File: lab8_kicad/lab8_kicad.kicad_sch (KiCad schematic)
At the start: 24 parts, among them J1 Command Generator, M1 Motor, SW1 Reset, U1 SN754410, U2 PIC32MX170F256B

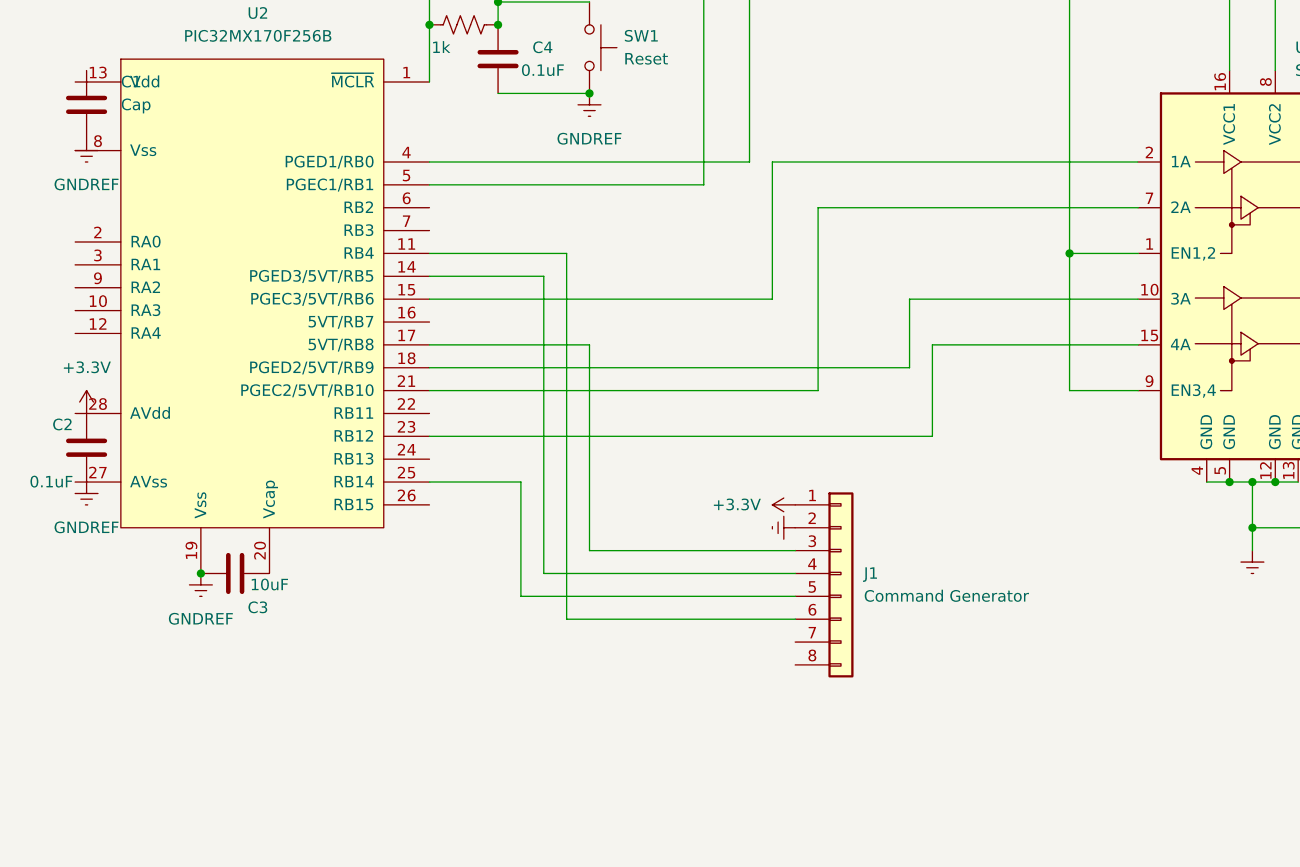
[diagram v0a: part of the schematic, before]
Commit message: suibian
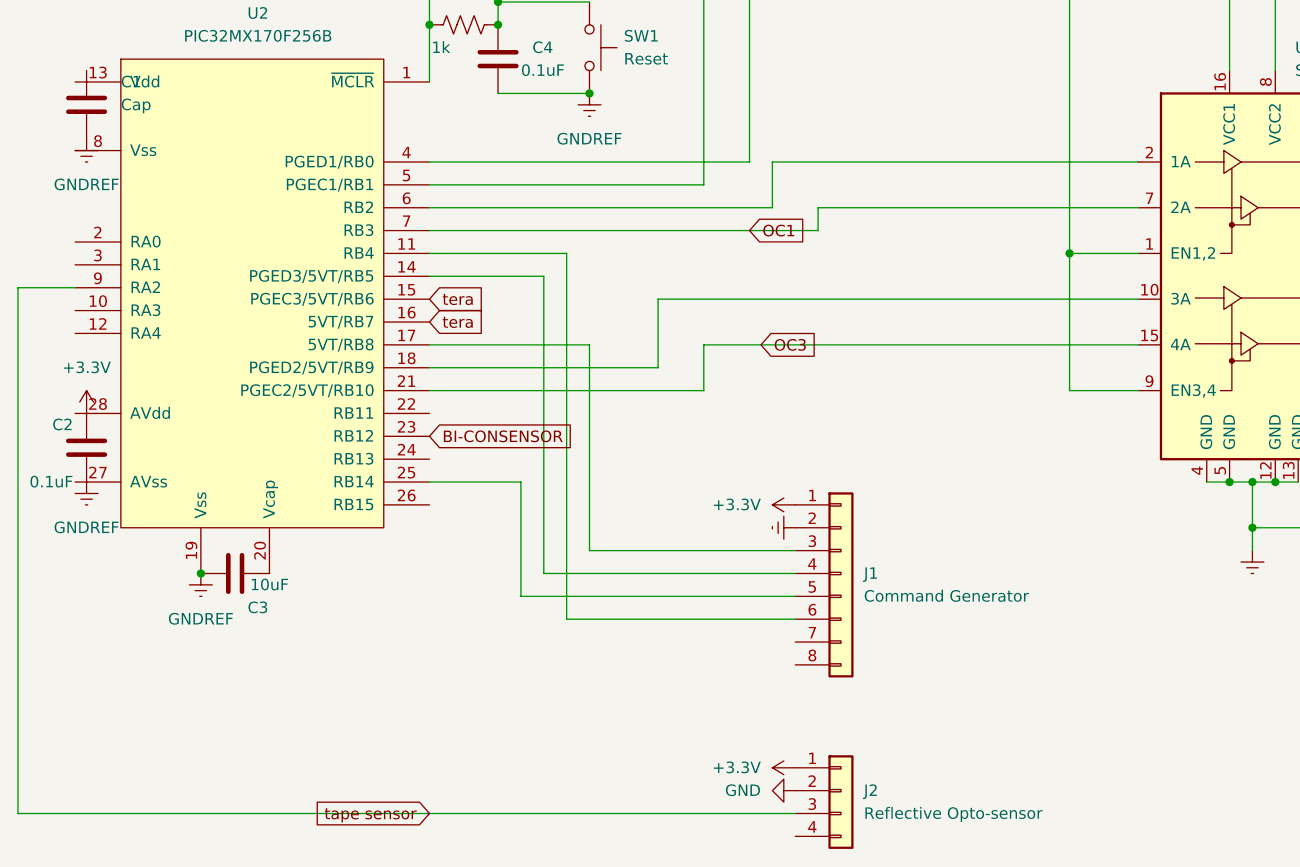
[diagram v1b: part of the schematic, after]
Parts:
- added J2: Reflective Opto-sensor, symbol ME218_BaseLib:Molex4
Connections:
- net +3.3V: now also J2.1 (Pin_1)
- net GND: now also J2.2 (Pin_2)
- net BI-CONSENSOR: now reaches U2.23 (RB12)
- net BI-CONSENSOR: no longer U1.15 (4A)
- net at U1.2 (1A): now also U2.6 (RB2); no longer U2.15 (PGEC3/5VT/RB6)
- net OC1: now reaches U1.7 (2A)
- net OC1: now also U2.7 (RB3); no longer U2.21 (PGEC2/5VT/RB10)
- net tera: now reaches U2.16 (5VT/RB7)
- net tera: now also U2.15 (PGEC3/5VT/RB6)
- net tape sensor: now reaches U2.9 (RA2)
- net tape sensor: now also J2.3 (Pin_3)
- new net OC3: U1.15 (4A), U2.21 (PGEC2/5VT/RB10)
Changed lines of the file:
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@@
+    (stroke (width 0) (type default))
+  )
+  (wire (pts (xy 104.14 60.96) (xy 66.04 60.96))
+    (stroke (width 0) (type default))
+  )
+  (wire (pts (xy 104.14 55.88) (xy 104.14 60.96))
     (stroke (width 0) (type default))
   )
@@
     (stroke (width 0) (type default))
   )
-  (wire (pts (xy 104.14 55.88) (xy 104.14 71.12))
-    (stroke (width 0) (type default))
-  )
   (wire (pts (xy 210.82 38.1) (xy 210.82 76.2))
     (stroke (width 0) (type default))
@@
     (stroke (width 0) (type default))
   )
+  (wire (pts (xy 109.22 63.5) (xy 66.04 63.5))
+    (stroke (width 0) (type default))
+  )
   (wire (pts (xy 256.54 91.44) (xy 269.24 91.44))
     (stroke (width 0) (type default))
   )
-  (wire (pts (xy 109.22 60.96) (xy 109.22 81.28))
-    (stroke (width 0) (type default))
-  )
   (wire (pts (xy 259.08 68.58) (xy 271.78 68.58))
     (stroke (width 0) (type default))
   )
-  (wire (pts (xy 66.04 71.12) (xy 104.14 71.12))
-    (stroke (width 0) (type default))
-  )
   (wire (pts (xy 73.66 38.1) (xy 83.82 38.1))
     (stroke (width 0) (type default))
@@
     (stroke (width 0) (type default))
   )
-  (wire (pts (xy 121.92 86.36) (xy 121.92 76.2))
+  (wire (pts (xy 96.52 81.28) (xy 66.04 81.28))
+    (stroke (width 0) (type default))
+  )
+  (wire (pts (xy 20.32 128.27) (xy 20.32 69.85))
+    (stroke (width 0) (type default))
+  )
+  (wire (pts (xy 96.52 76.2) (xy 96.52 81.28))
     (stroke (width 0) (type default))
   )
@@
     (stroke (width 0) (type default))
   )
-  (wire (pts (xy 119.38 78.74) (xy 119.38 71.12))
-    (stroke (width 0) (type default))
-  )
-  (wire (pts (xy 121.92 76.2) (xy 144.78 76.2))
-    (stroke (width 0) (type default))
-  )
-  (wire (pts (xy 119.38 71.12) (xy 144.78 71.12))
+  (wire (pts (xy 91.44 78.74) (xy 66.04 78.74))
     (stroke (width 0) (type default))
   )
@@
     (stroke (width 0) (type default))
   )
+  (wire (pts (xy 20.32 69.85) (xy 26.67 69.85))
+    (stroke (width 0) (type default))
+  )
   (wire (pts (xy 144.78 66.04) (xy 137.16 66.04))
     (stroke (width 0) (type default))
@@
     (stroke (width 0) (type default))
   )
-  (wire (pts (xy 66.04 86.36) (xy 121.92 86.36))
+  (wire (pts (xy 106.68 128.27) (xy 20.32 128.27))
     (stroke (width 0) (type default))
   )
@@
     (stroke (width 0) (type default))
   )
+  (wire (pts (xy 144.78 76.2) (xy 96.52 76.2))
+    (stroke (width 0) (type default))
+  )
   (wire (pts (xy 243.84 25.4) (xy 248.92 25.4))
     (stroke (width 0) (type default))
@@
     (stroke (width 0) (type default))
   )
+  (wire (pts (xy 144.78 71.12) (xy 91.44 71.12))
+    (stroke (width 0) (type default))
+  )
   (wire (pts (xy 193.04 38.1) (xy 193.04 60.96))
     (stroke (width 0) (type default))
@@
     (stroke (width 0) (type default))
   )
-  (wire (pts (xy 66.04 81.28) (xy 109.22 81.28))
-    (stroke (width 0) (type default))
-  )
-  (wire (pts (xy 66.04 78.74) (xy 119.38 78.74))
+  (wire (pts (xy 91.44 71.12) (xy 91.44 78.74))
+    (stroke (width 0) (type default))
+  )
+  (wire (pts (xy 109.22 60.96) (xy 109.22 63.5))
     (stroke (width 0) (type default))
   )
@@
   (text "RIGHT Motor" (at 262.89 49.53 0)
     (effects (font (size 1.27 1.27)) (justify left bottom))
+  )
+  (global_label "tera" (shape input) (at 66.04 71.12 0) (fields_autoplaced)
+    (effects (font (size 1.27 1.27)) (justify left))
+    (property "Intersheetrefs" "${INTERSHEET_REFS}" (at 72.7747 71.12 0)
+      (effects (font (size 1.27 1.27)) (justify left) hide)
+    )
+  )
+  (global_label "OC3" (shape input) (at 102.87 76.2 0) (fields_autoplaced)
+    (effects (font (size 1.27 1.27)) (justify left))
+    (property "Intersheetrefs" "${INTERSHEET_REFS}" (at 109.6652 76.2 0)
+      (effects (font (size 1.27 1.27)) (justify left) hide)
+    )
+  )
+  (global_label "tape sensor" (shape input) (at 66.04 128.27 180) (fields_autoplaced)
+    (effects (font (size 1.27 1.27)) (justify right))
+    (property "Intersheetrefs" "${INTERSHEET_REFS}" (at 51.7459 128.27 0)
+      (effects (font (size 1.27 1.27)) (justify right) hide)
+    )
+  )
+  (global_label "BI-CONSENSOR" (shape input) (at 66.04 86.36 0) (fields_autoplaced)
+    (effects (font (size 1.27 1.27)) (justify left))
+    (property "Intersheetrefs" "${INTERSHEET_REFS}" (at 83.9024 86.36 0)
+      (effects (font (size 1.27 1.27)) (justify left) hide)
+    )
+  )
+  (global_label "tera" (shape input) (at 66.04 73.66 0) (fields_autoplaced)
+    (effects (font (size 1.27 1.27)) (justify left))
+    (property "Intersheetrefs" "${INTERSHEET_REFS}" (at 72.7747 73.66 0)
+      (effects (font (size 1.27 1.27)) (justify left) hide)
+    )
+  )
+  (global_label "OC1" (shape input) (at 101.6 63.5 0) (fields_autoplaced)
+    (effects (font (size 1.27 1.27)) (justify left))
+    (property "Intersheetrefs" "${INTERSHEET_REFS}" (at 108.3952 63.5 0)
+      (effects (font (size 1.27 1.27)) (justify left) hide)
+    )
   )
   (symbol (lib_id "ME218_BaseLib:SW_Push") (at 83.82 43.18 270) (unit 1)
@@
         (path "/c54286ed-3a82-4325-b913-88d6215d969b"
           (reference "D1") (unit 1)
+        )
+      )
+    )
+  )
+  (symbol (lib_id "power:+3.3V") (at 106.68 123.19 90) (unit 1)
+    (in_bom yes) (on_board yes) (dnp no) (fields_autoplaced)
+    (property "Reference" "#PWR09" (at 110.49 123.19 0)
+      (effects (font (size 1.27 1.27)) hide)
+    )
+    (property "Value" "+3.3V" (at 102.87 123.19 90)
+      (effects (font (size 1.27 1.27)) (justify left))
+    )
+    (property "Footprint" "" (at 106.68 123.19 0)
+      (effects (font (size 1.27 1.27)) hide)
+    )
+    (property "Datasheet" "" (at 106.68 123.19 0)
+      (effects (font (size 1.27 1.27)) hide)
+    )
+    (pin "1")
+    (instances
+      (project "lab8_kicad"
+        (path "/c3d935fb-33dd-45da-8182-93745821b586"
+          (reference "#PWR09") (unit 1)
         )
       )
@@
     )
   )
+  (symbol (lib_id "ME218_BaseLib:Molex4") (at 111.76 125.73 0) (unit 1)
+    (in_bom yes) (on_board yes) (dnp no) (fields_autoplaced)
+    (property "Reference" "J2" (at 114.3 125.73 0)
+      (effects (font (size 1.27 1.27)) (justify left))
+    )
+    (property "Value" "Reflective Opto-sensor" (at 114.3 128.27 0)
+      (effects (font (size 1.27 1.27)) (justify left))
+    )
+    (property "Footprint" "" (at 111.76 125.73 0)
+      (effects (font (size 1.27 1.27)) hide)
+    )
+    (property "Datasheet" "" (at 111.76 125.73 0)
+      (effects (font (size 1.27 1.27)) hide)
+    )
+    (pin "1")
+    (pin "2")
+    (pin "3")
+    (pin "4")
+    (instances
+      (project "lab8_kicad"
+        (path "/c3d935fb-33dd-45da-8182-93745821b586"
+          (reference "J2") (unit 1)
+        )
+      )
+    )
+  )
   (symbol (lib_id "ME218_BaseLib:LED") (at 240.03 25.4 0) (unit 1)
     (in_bom yes) (on_board yes) (dnp no) (fields_autoplaced)
@@
         )
       )
+    )
+  )
+  (symbol (lib_id "power:GND") (at 106.68 125.73 270) (unit 1)
+    (in_bom yes) (on_board yes) (dnp no) (fields_autoplaced)
+    (property "Reference" "#PWR010" (at 100.33 125.73 0)
+      (effects (font (size 1.27 1.27)) hide)
+    )
+    (property "Value" "GND" (at 102.87 125.73 90)
+      (effects (font (size 1.27 1.27)) (justify right))
+    )
+    (property "Footprint" "" (at 106.68 125.73 0)
+      (effects (font (size 1.27 1.27)) hide)
+    )
+    (property "Datasheet" "" (at 106.68 125.73 0)
+      (effects (font (size 1.27 1.27)) hide)
+    )
+    (pin "1")
+    (instances
+      (project "lab8_kicad"
+        (path "/c3d935fb-33dd-45da-8182-93745821b586"
+          (reference "#PWR010") (unit 1)
+        )
+      )

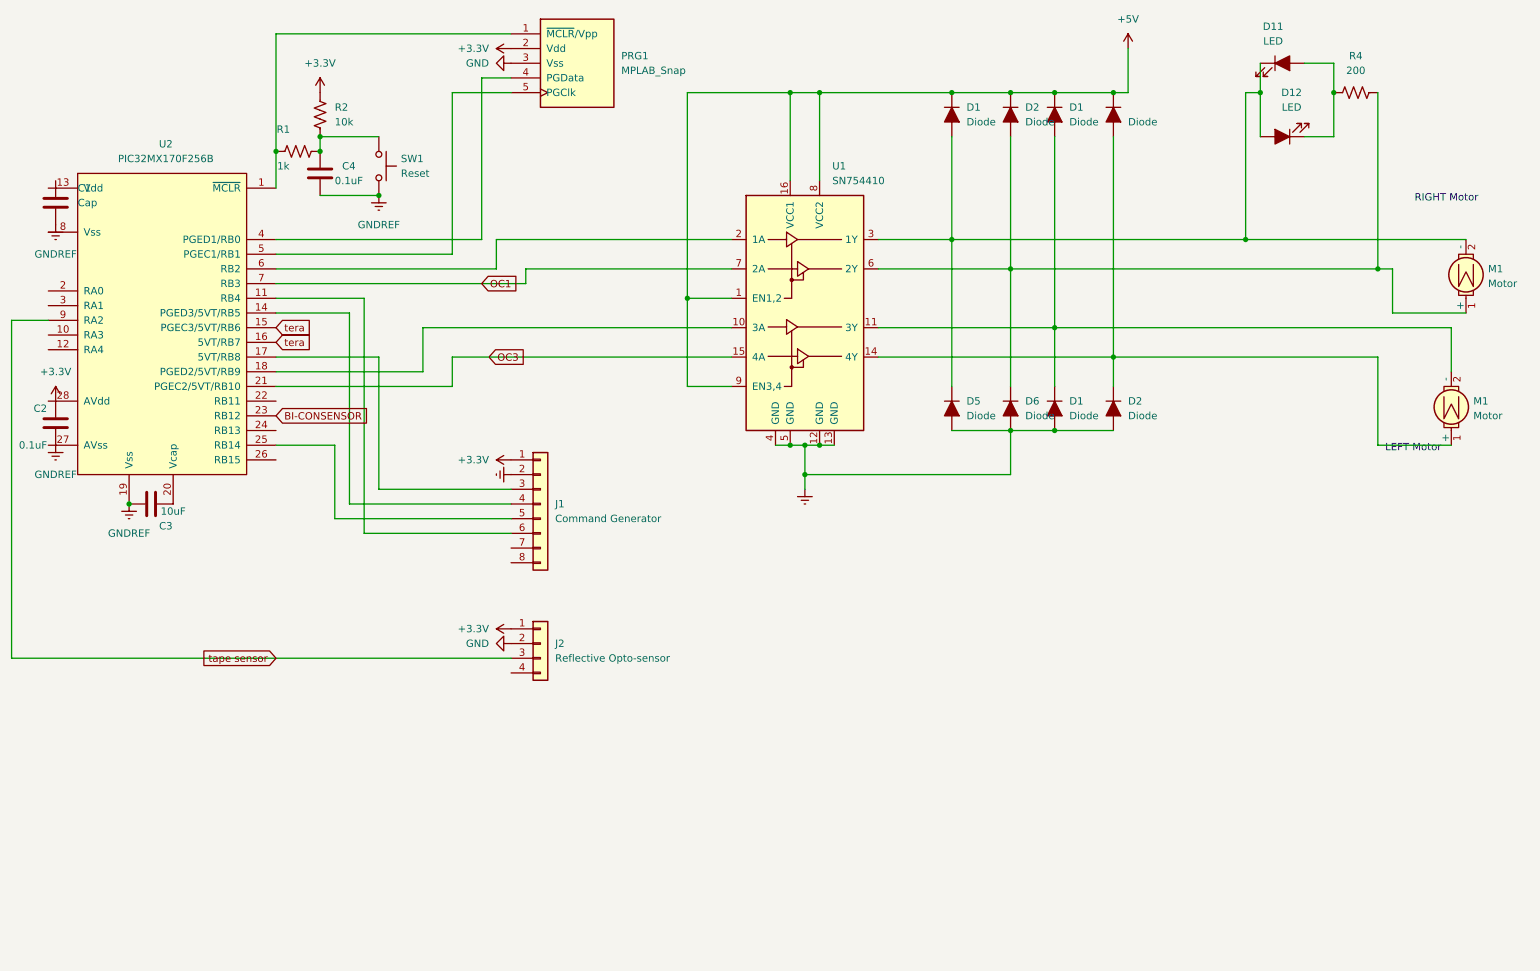
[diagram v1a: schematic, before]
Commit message: fix schemetic
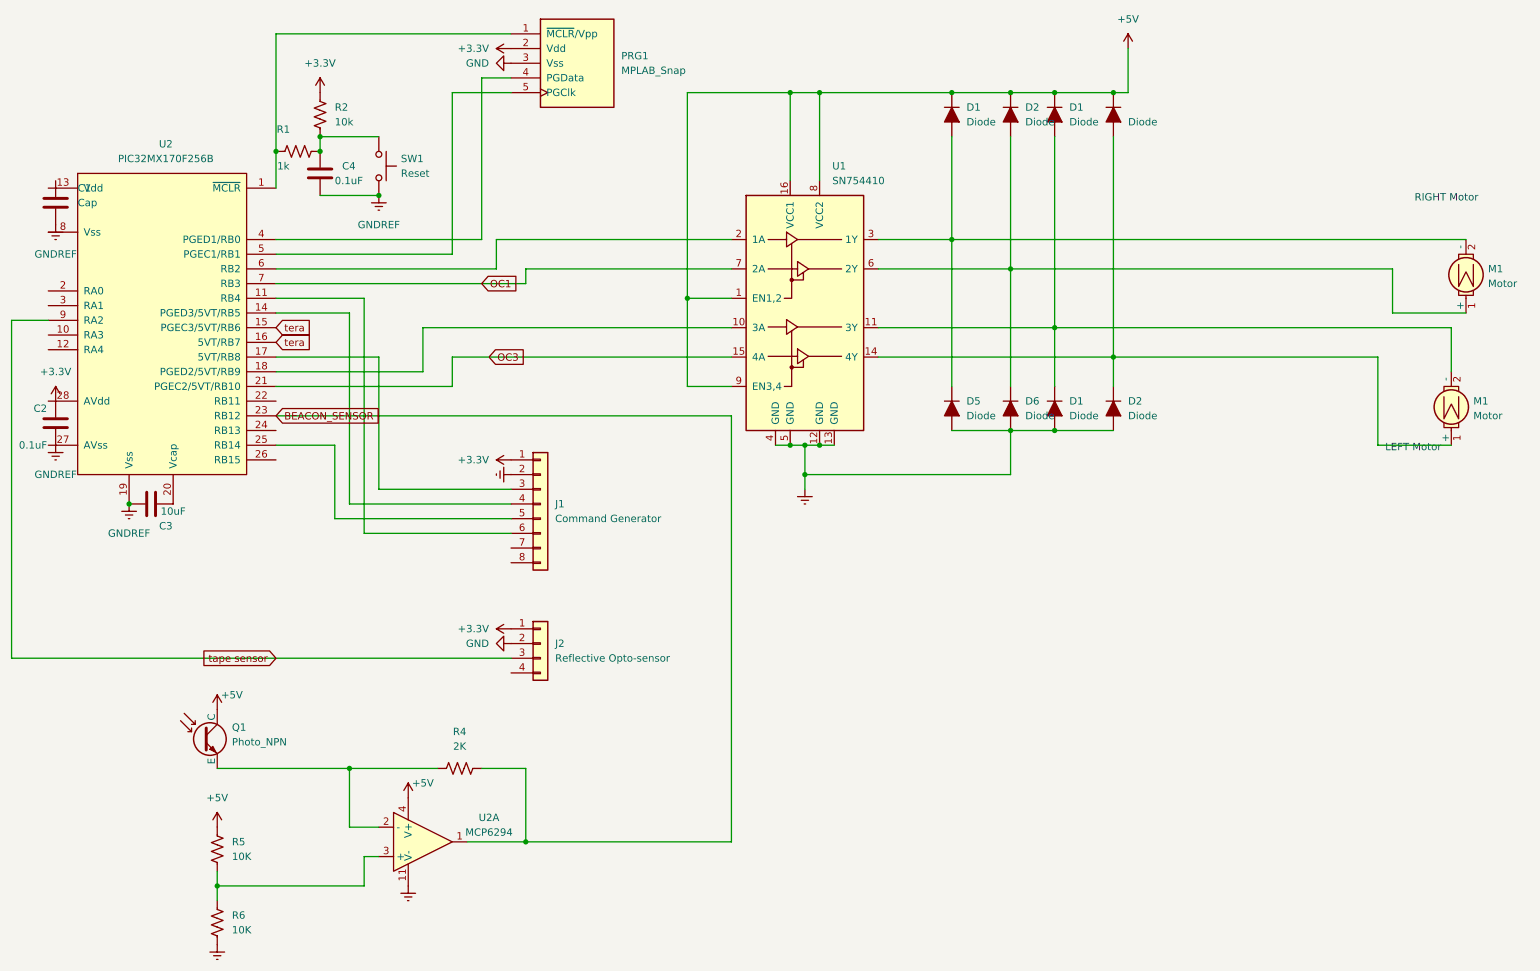
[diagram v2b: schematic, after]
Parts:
- removed D11, D12: LED, symbol ME218_BaseLib:LED
- added Q1: Photo_NPN, symbol ME218_BaseLib:Photo_NPN
- added R5, R6: 10K, symbol ME218_BaseLib:Res1
- added U2: MCP6294, symbol ME218_BaseLib:MCP6294
- R4: value 200 -> 2K
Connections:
- net +5V: now also Q1.1 (C), R5.1, U2.4 (V+)
- net Earth: now also R6.2, U2.11 (V-)
- net at R4.1: now also Q1.2 (E), U2.2 (-)
- net at D2.2 (A), D6.1 (K), M1.1 (+)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: no longer R4.2
- net BI-CONSENSOR renamed BEACON_SENSOR
- net BEACON_SENSOR: now also R4.2, U2.1
- new net: R5.2, R6.1, U2.3 (+)
